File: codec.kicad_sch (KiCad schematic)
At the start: 16 parts, among them J1 Conn_01x03_Pin, U2 CM108AH, U3 93C46

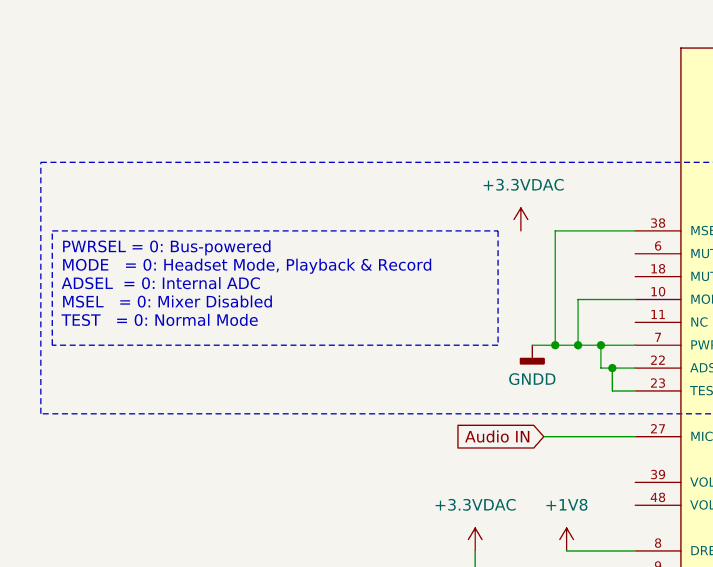
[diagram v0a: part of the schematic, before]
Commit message: kiCAD 9.0
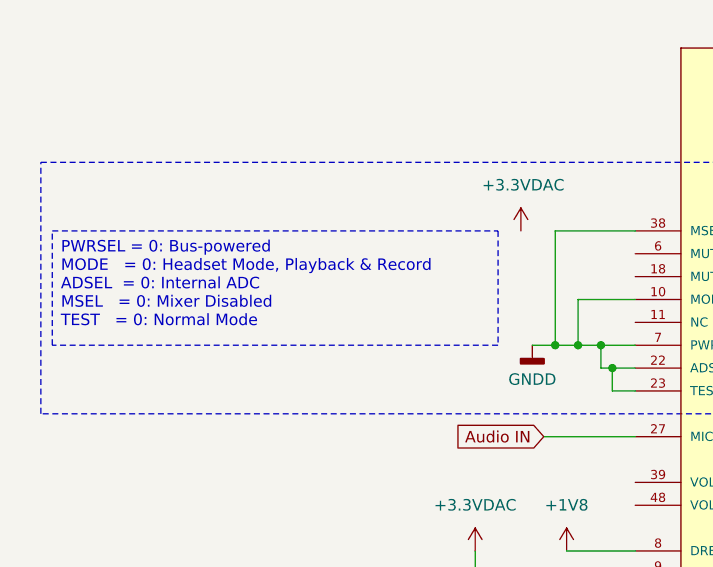
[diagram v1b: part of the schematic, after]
